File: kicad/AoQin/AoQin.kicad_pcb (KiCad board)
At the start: 2 copper layers, 113.5 x 83 mm, 17 parts, among them J1 Conn_01x03_Socket, J10 1985218, J12 1985218, J2 Conn_01x03_Socket, J3 Conn_02x03_Odd_Even, J4 Conn_02x03_Odd_Even, J5 1985218, J6 1985218, J8 1985218, J9 1985218

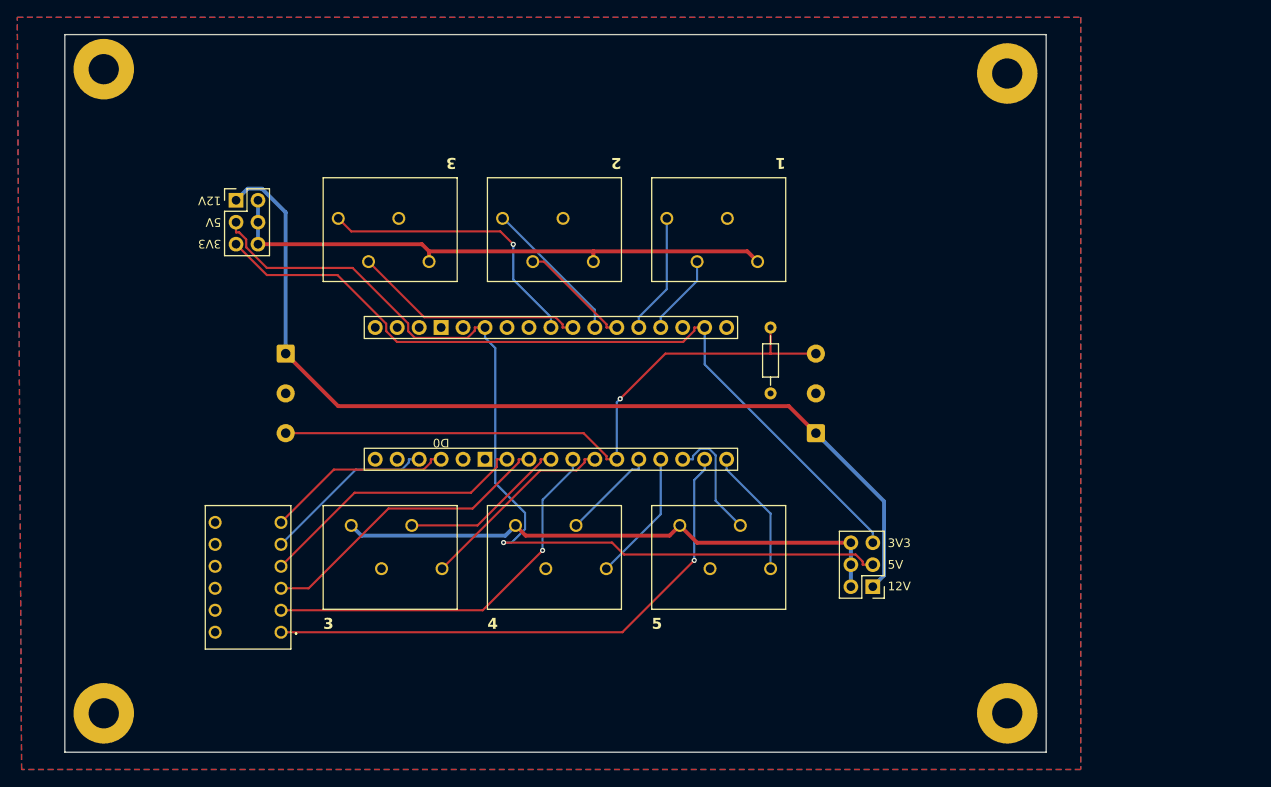
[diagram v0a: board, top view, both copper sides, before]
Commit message: The Reckoning
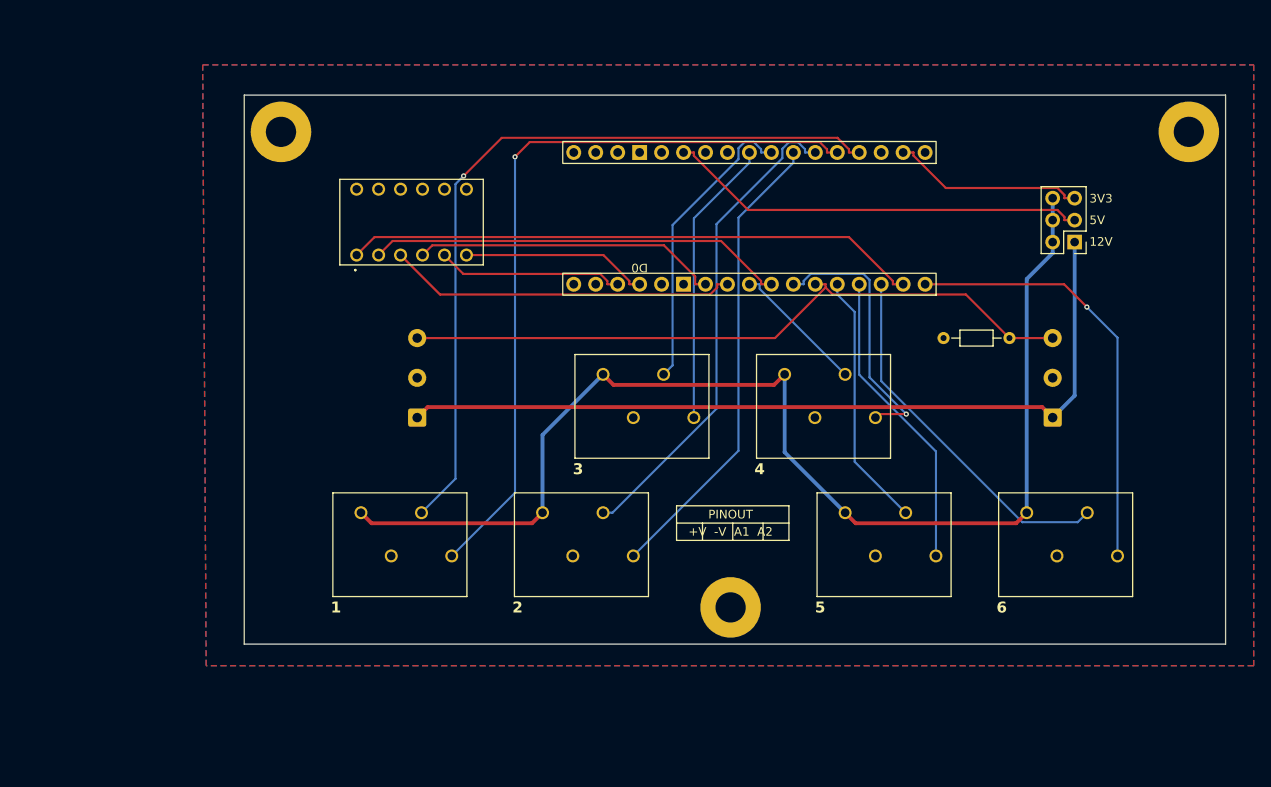
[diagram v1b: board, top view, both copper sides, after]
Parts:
- removed H4: MountingHole_Pad, MountingHole:MountingHole_3.5mm_Pad
- removed J4: Conn_02x03_Odd_Even, Connector_PinHeader_2.54mm:PinHeader_2x03_P2.54mm_Vertical
- moved J10 75.0 mm to (142.6, 71.8), turned to 0 degrees
- moved J3 46.2 mm to (148.1, 40.5)
- moved S2 44.5 mm to (65.1, 42.0), turned to 0 degrees
- moved H3 34.3 mm to (108.3, 82.7)
- moved A1 30.6 mm to (134.8, 28.7)
- moved R13 27.7 mm to (140.6, 51.6), turned to 180 degrees
- moved J1 27.4 mm to (145.6, 60.8)
- moved J9 25.7 mm to (114.6, 55.8), turned to 0 degrees
- moved J8 22.1 mm to (93.6, 55.8), turned to 0 degrees
- moved H2 22.1 mm to (161.3, 27.7)
- moved H1 21.7 mm to (56.3, 27.7)
- moved J12 19.2 mm to (121.6, 71.8)
- moved J2 16.9 mm to (72.1, 60.8), turned to 90 degrees
- moved J6 3.45 mm to (86.6, 71.8)
- moved J5 1.85 mm to (65.6, 71.8)
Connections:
- J10 pad 1: /VIN2 -> /VIN
- J10 pad 3: /A4 -> /A10
- J10 pad 4: /A5 -> /A11
- J12 pad 1: /VIN1 -> /VIN
- J12 pad 3: /A10 -> /A8
- J12 pad 4: /A11 -> /A9
- J3 pad 2: /VIN1 -> /VIN
- J3 pad 4: /VIN1 -> /VIN
- J3 pad 6: /VIN1 -> /VIN
- J5 pad 1: /VIN1 -> /VIN
- J5 pad 3: /A6 -> /A0
- J5 pad 4: /A7 -> /A1
- J6 pad 1: /VIN1 -> /VIN
- J6 pad 3: /A8 -> /A2
- J6 pad 4: /A9 -> /A3
- J8 pad 1: /VIN2 -> /VIN
- J8 pad 3: /A0 -> /A4
- J8 pad 4: /A1 -> /A5
- J9 pad 1: /VIN2 -> /VIN
- J9 pad 3: /A2 -> /A6
- J9 pad 4: /A3 -> /A7
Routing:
- net /VIN: track 0.00 -> 141.4 mm
- net /A0: track 9.36 -> 89.5 mm, vias 0 -> 1
- net /A1: track 14.0 -> 87.9 mm, vias 0 -> 1
- net /3V3: track 93.2 -> 22.5 mm
- net /VIN2: track 66.1 -> 0.00 mm
- net /VIN1: track 65.6 -> 0.00 mm
- net /5V: track 109.2 -> 48.9 mm, vias 1 -> 0
- net /A2: track 13.1 -> 56.2 mm
- net /A3: track 17.1 -> 54.3 mm
- net /A11: track 14.8 -> 50.1 mm, vias 0 -> 1
- net /A10: track 14.1 -> 42.2 mm
- net /A9: track 15.3 -> 35.1 mm
- net /A8: track 11.1 -> 29.7 mm
- net +12V: track 110.5 -> 95.9 mm
- net /A7: track 23.1 -> 30.8 mm, vias 0 -> 1
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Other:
- board size 113.5 x 83 mm -> 113.5 x 63.5 mm
- board text added: "+V -V A1 A2"
- board text added: "6"
- board text added: "PINOUT"

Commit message: Prometheus
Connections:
- A1 pad VIN: /VCC -> +12V
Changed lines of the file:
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@@
 	(net 29 "/A11")
 	(net 30 "/A2")
-	(net 31 "/VCC")
-	(net 32 "/A7")
-	(net 33 "/A6")
+	(net 31 "/A7")
+	(net 32 "/A6")
 	(footprint "Connector_Wire:SolderWire-0.5sqmm_1x03_P4.6mm_D0.9mm_OD2.1mm"
 		(layer "F.Cu")
@@
 			(layers "*.Cu" "*.Mask")
 			(remove_unused_layers no)
-			(net 33 "/A6")
+			(net 32 "/A6")
 			(pinfunction "D4")
 			(pintype "bidirectional")
@@
 			(layers "*.Cu" "*.Mask")
 			(remove_unused_layers no)
-			(net 32 "/A7")
+			(net 31 "/A7")
 			(pinfunction "D6")
 			(pintype "bidirectional")
@@
 			(layers "*.Cu" "*.Mask")
 			(remove_unused_layers no)
-			(net 31 "/VCC")
+			(net 17 "+12V")
 			(pinfunction "VIN")
 			(pintype "power_in")
@@
 			(layers "*.Cu" "*.Mask")
 			(remove_unused_layers no)
-			(net 33 "/A6")
+			(net 32 "/A6")
 			(pinfunction "3")
 			(pintype "passive")
@@
 			(layers "*.Cu" "*.Mask")
 			(remove_unused_layers no)
-			(net 32 "/A7")
+			(net 31 "/A7")
 			(pinfunction "4")
 			(pintype "passive")
@@
 		(width 0.25)
 		(layer "F.Cu")
-		(net 32)
+		(net 31)
 	)
 	(segment
@@
 		(width 0.25)
 		(layer "F.Cu")
-		(net 32)
+		(net 31)
 	)
 	(via
@@
 		(drill 0.3)
 		(layers "F.Cu" "B.Cu")
-		(net 32)
+		(net 31)
 	)
 	(segment
@@
 		(width 0.25)
 		(layer "B.Cu")
-		(net 32)
+		(net 31)
 	)
 	(segment
@@
 		(width 0.25)
 		(layer "B.Cu")
-		(net 32)
+		(net 31)
 	)
 	(segment
@@
 		(width 0.25)
 		(layer "B.Cu")
-		(net 32)
+		(net 31)
 	)
 	(segment
@@
 		(width 0.25)
 		(layer "B.Cu")
-		(net 32)
+		(net 31)
 	)
 	(segment
@@
 		(width 0.25)
 		(layer "B.Cu")
-		(net 32)
+		(net 31)
 	)
 	(segment
@@
 		(width 0.25)
 		(layer "B.Cu")
-		(net 32)
+		(net 31)
 	)
 	(segment
@@
 		(width 0.25)
 		(layer "B.Cu")
-		(net 32)
+		(net 31)
 	)
 	(segment
@@
 		(width 0.25)
 		(layer "B.Cu")
-		(net 33)
+		(net 32)
 	)
 	(segment
@@
 		(width 0.25)
 		(layer "B.Cu")
-		(net 33)
+		(net 32)
 	)
 	(segment
@@
 		(width 0.25)
 		(layer "B.Cu")
-		(net 33)
+		(net 32)
 	)
 	(zone
